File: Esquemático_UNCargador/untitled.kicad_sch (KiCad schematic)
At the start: 8 parts

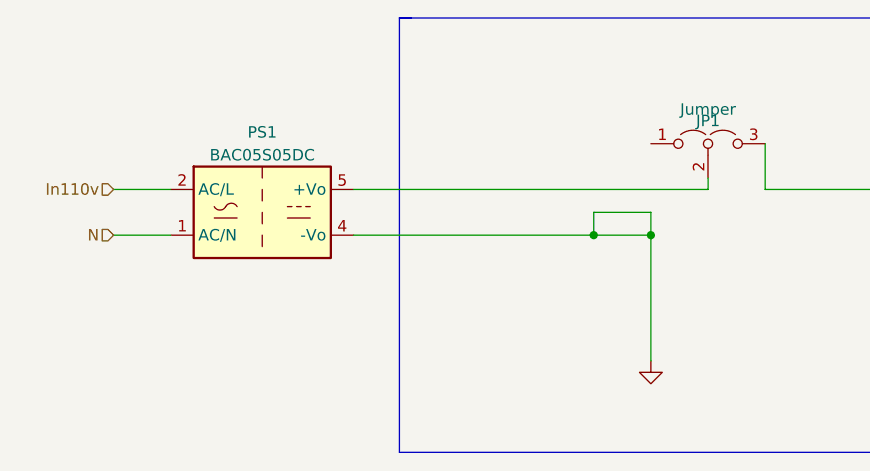
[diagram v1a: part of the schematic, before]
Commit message: version inicial layout PCB
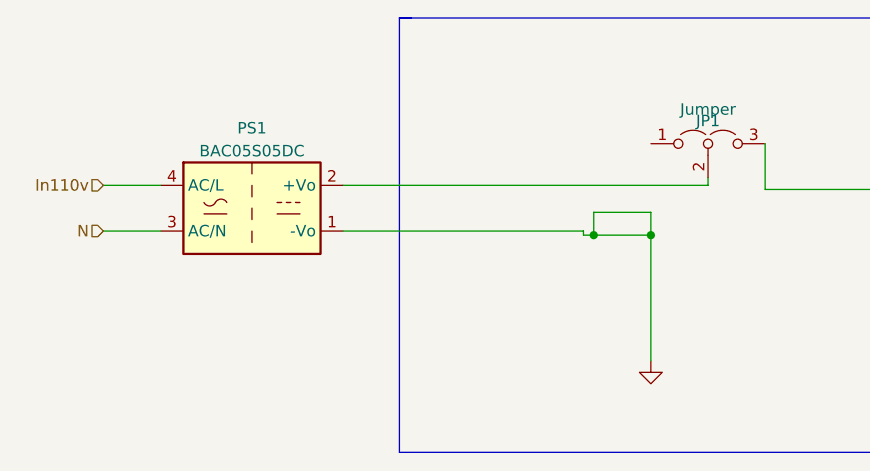
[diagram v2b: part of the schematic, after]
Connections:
- net GND: now also PS1.1 (-Vo); no longer PS1.4 (-Vo)
- net In110v: now also PS1.4 (AC/L); no longer PS1.2 (AC/L)
- net N: now also PS1.3 (NC); no longer PS1.1 (AC/N)
- net at JP1.2 (C): now also PS1.2 (+Vo); no longer PS1.5 (+Vo)
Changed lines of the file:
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@@
     (stroke (width 0) (type default))
   )
-  (wire (pts (xy 59.563 90.6272) (xy 98.933 90.6272))
+  (wire (pts (xy 58.42 90.17) (xy 98.933 90.17))
     (stroke (width 0) (type default))
   )
@@
     (stroke (width 0) (type default))
   )
-  (wire (pts (xy 32.893 95.7072) (xy 39.243 95.7072))
-    (stroke (width 0) (type default))
-  )
-  (wire (pts (xy 98.933 89.3572) (xy 98.933 90.6272))
+  (wire (pts (xy 31.75 95.25) (xy 38.1 95.25))
+    (stroke (width 0) (type default))
+  )
+  (wire (pts (xy 98.933 89.3572) (xy 98.933 90.17))
     (stroke (width 0) (type default))
   )
@@
     (stroke (width 0) (type default))
   )
-  (wire (pts (xy 59.563 95.7072) (xy 86.233 95.7072))
+  (wire (pts (xy 58.42 95.25) (xy 85.09 95.25))
     (stroke (width 0) (type default))
   )
@@
     (stroke (width 0) (type default))
   )
-  (wire (pts (xy 32.893 90.6272) (xy 39.243 90.6272))
+  (wire (pts (xy 31.75 90.17) (xy 38.1 90.17))
     (stroke (width 0) (type default))
   )
@@
     (stroke (width 0) (type default))
   )
+  (wire (pts (xy 85.09 95.7072) (xy 86.233 95.7072))
+    (stroke (width 0) (type default))
+  )
   (wire (pts (xy 107.0356 143.0274) (xy 107.0356 155.7274))
     (stroke (width 0) (type default))
@@
   )
   (wire (pts (xy 105.283 90.6272) (xy 142.113 90.6272))
+    (stroke (width 0) (type default))
+  )
+  (wire (pts (xy 85.09 95.25) (xy 85.09 95.7072))
     (stroke (width 0) (type default))
   )
@@
     (effects (font (size 1.27 1.27)) (justify left bottom))
   )
-  (hierarchical_label "In110v" (shape input) (at 32.893 90.6272 180) (fields_autoplaced)
+  (hierarchical_label "In110v" (shape input) (at 31.75 90.17 180) (fields_autoplaced)
     (effects (font (size 1.27 1.27)) (justify right))
   )
-  (hierarchical_label "N" (shape input) (at 32.893 95.7072 180) (fields_autoplaced)
+  (hierarchical_label "N" (shape input) (at 31.75 95.25 180) (fields_autoplaced)
     (effects (font (size 1.27 1.27)) (justify right))
   )
@@
         (path "/f64e4c48-29c2-4644-b6e3-d55b9152fc29/c38372d7-094a-4ec0-82ac-c3a161d378bf"
           (reference "#PWR0122") (unit 1)
-        )
-      )
-    )
-  )
-  (symbol (lib_id "Converter_ACDC:BAC05S05DC") (at 49.403 93.1672 0) (unit 1)
-    (in_bom yes) (on_board yes) (dnp no) (fields_autoplaced)
-    (property "Reference" "PS1" (at 49.403 84.2772 0)
-      (effects (font (size 1.27 1.27)))
-    )
-    (property "Value" "BAC05S05DC" (at 49.403 86.8172 0)
-      (effects (font (size 1.27 1.27)))
-    )
-    (property "Footprint" "Convertidor_AC-DC:AC-DC_Converter" (at 49.403 102.0572 0)
-      (effects (font (size 1.27 1.27)) hide)
-    )
-    (property "Datasheet" "" (at 49.403 104.5972 0)
-      (effects (font (size 1.27 1.27)) hide)
-    )
-    (pin "1")
-    (pin "2")
-    (pin "3")
-    (pin "4")
-    (pin "5")
-    (instances
-      (project "untitled"
-        (path "/9be105a0-504f-4b07-b004-211a0f61b6b4"
-          (reference "PS1") (unit 1)
-        )
-      )
-      (project "CircuitoPotencia"
-        (path "/f64e4c48-29c2-4644-b6e3-d55b9152fc29/c38372d7-094a-4ec0-82ac-c3a161d378bf"
-          (reference "PS1") (unit 1)
         )
       )
@@
       (project "CircuitoPotencia"
         (path "/f64e4c48-29c2-4644-b6e3-d55b9152fc29/c38372d7-094a-4ec0-82ac-c3a161d378bf"
-          (reference "U_5V") (unit 1)
+          (reference "U_5V1") (unit 1)
         )
       )
@@
       (project "CircuitoPotencia"
         (path "/f64e4c48-29c2-4644-b6e3-d55b9152fc29/c38372d7-094a-4ec0-82ac-c3a161d378bf"
-          (reference "#PWR06") (unit 1)
+          (reference "#PWR0111") (unit 1)
         )
       )
@@
       (project "CircuitoPotencia"
         (path "/f64e4c48-29c2-4644-b6e3-d55b9152fc29/c38372d7-094a-4ec0-82ac-c3a161d378bf"
-          (reference "#PWR07") (unit 1)
+          (reference "#PWR0113") (unit 1)
         )
       )
@@
       (project "CircuitoPotencia"
         (path "/f64e4c48-29c2-4644-b6e3-d55b9152fc29/c38372d7-094a-4ec0-82ac-c3a161d378bf"
-          (reference "#PWR08") (unit 1)
+          (reference "#PWR0112") (unit 1)
         )
       )
@@
       (project "CircuitoPotencia"
         (path "/f64e4c48-29c2-4644-b6e3-d55b9152fc29/c38372d7-094a-4ec0-82ac-c3a161d378bf"
-          (reference "U_3.3V") (unit 1)
+          (reference "U_3.3V1") (unit 1)
         )
       )
@@
       (project "CircuitoPotencia"
         (path "/f64e4c48-29c2-4644-b6e3-d55b9152fc29/c38372d7-094a-4ec0-82ac-c3a161d378bf"
-          (reference "#PWR05") (unit 1)
+          (reference "#PWR0114") (unit 1)
         )
       )
@@
         )
       )
+    )
+  )
+  (symbol (lib_id "Converter_ACDC:BAC05S05DC") (at 48.26 92.71 0) (unit 1)
+    (in_bom yes) (on_board yes) (dnp no) (fields_autoplaced)
+    (property "Reference" "PS1" (at 48.26 83.82 0)
+      (effects (font (size 1.27 1.27)))
+    )
+    (property "Value" "BAC05S05DC" (at 48.26 86.36 0)
+      (effects (font (size 1.27 1.27)))
+    )
+    (property "Footprint" "Convertidor_AC-DC:AC-DC_Converter" (at 48.26 101.6 0)
+      (effects (font (size 1.27 1.27)) hide)
+    )
+    (property "Datasheet" "" (at 48.26 104.14 0)
+      (effects (font (size 1.27 1.27)) hide)
+    )
+    (pin "3")
+    (pin "4")
+    (pin "3")
+    (pin "1")
+    (pin "2")
+    (instances
+      (project "untitled"
+        (path "/9be105a0-504f-4b07-b004-211a0f61b6b4"
+          (reference "PS1") (unit 1)
+        )
+      )
+      (project "CircuitoPotencia"
+        (path "/f64e4c48-29c2-4644-b6e3-d55b9152fc29/c38372d7-094a-4ec0-82ac-c3a161d378bf"
+          (reference "PT1") (unit 1)
+        )
+        (path "/f64e4c48-29c2-4644-b6e3-d55b9152fc29/bcc2cbe9-78c8-42aa-91d0-1fe918a34d54"
+          (reference "PS1") (unit 1)
+        )
+      )
